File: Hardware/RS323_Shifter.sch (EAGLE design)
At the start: 16 parts, among them U2 XN04312

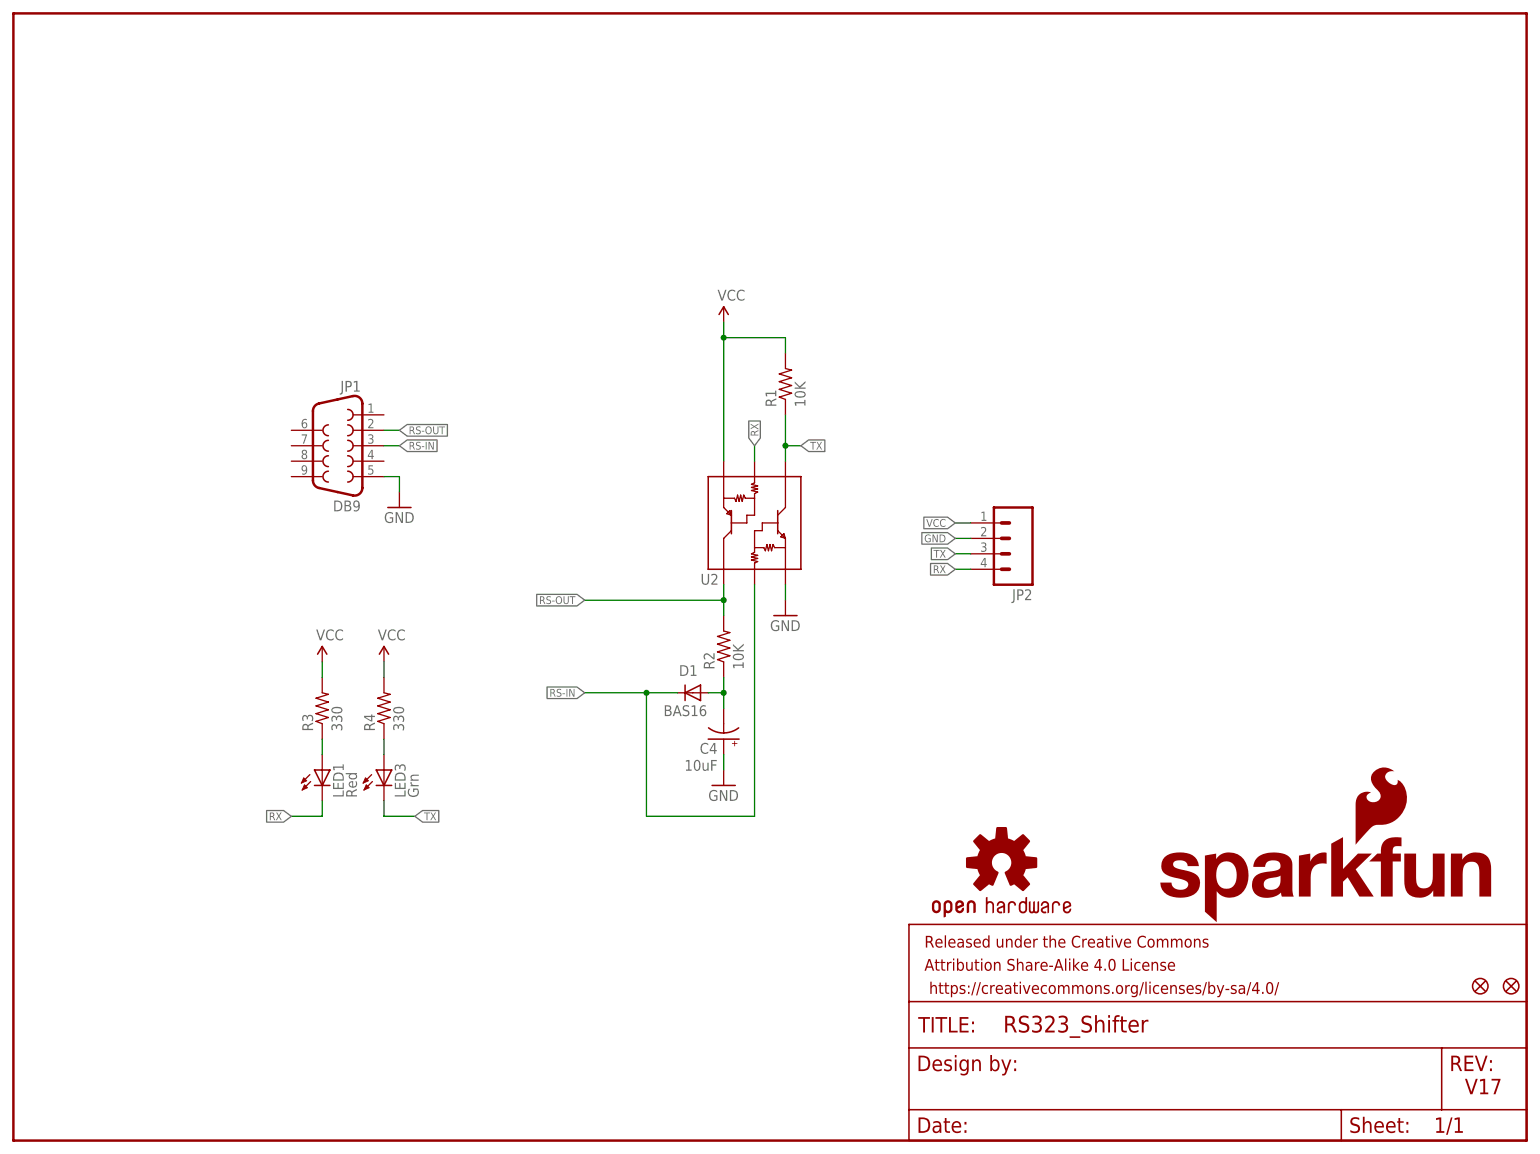
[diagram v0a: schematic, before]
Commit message: New files
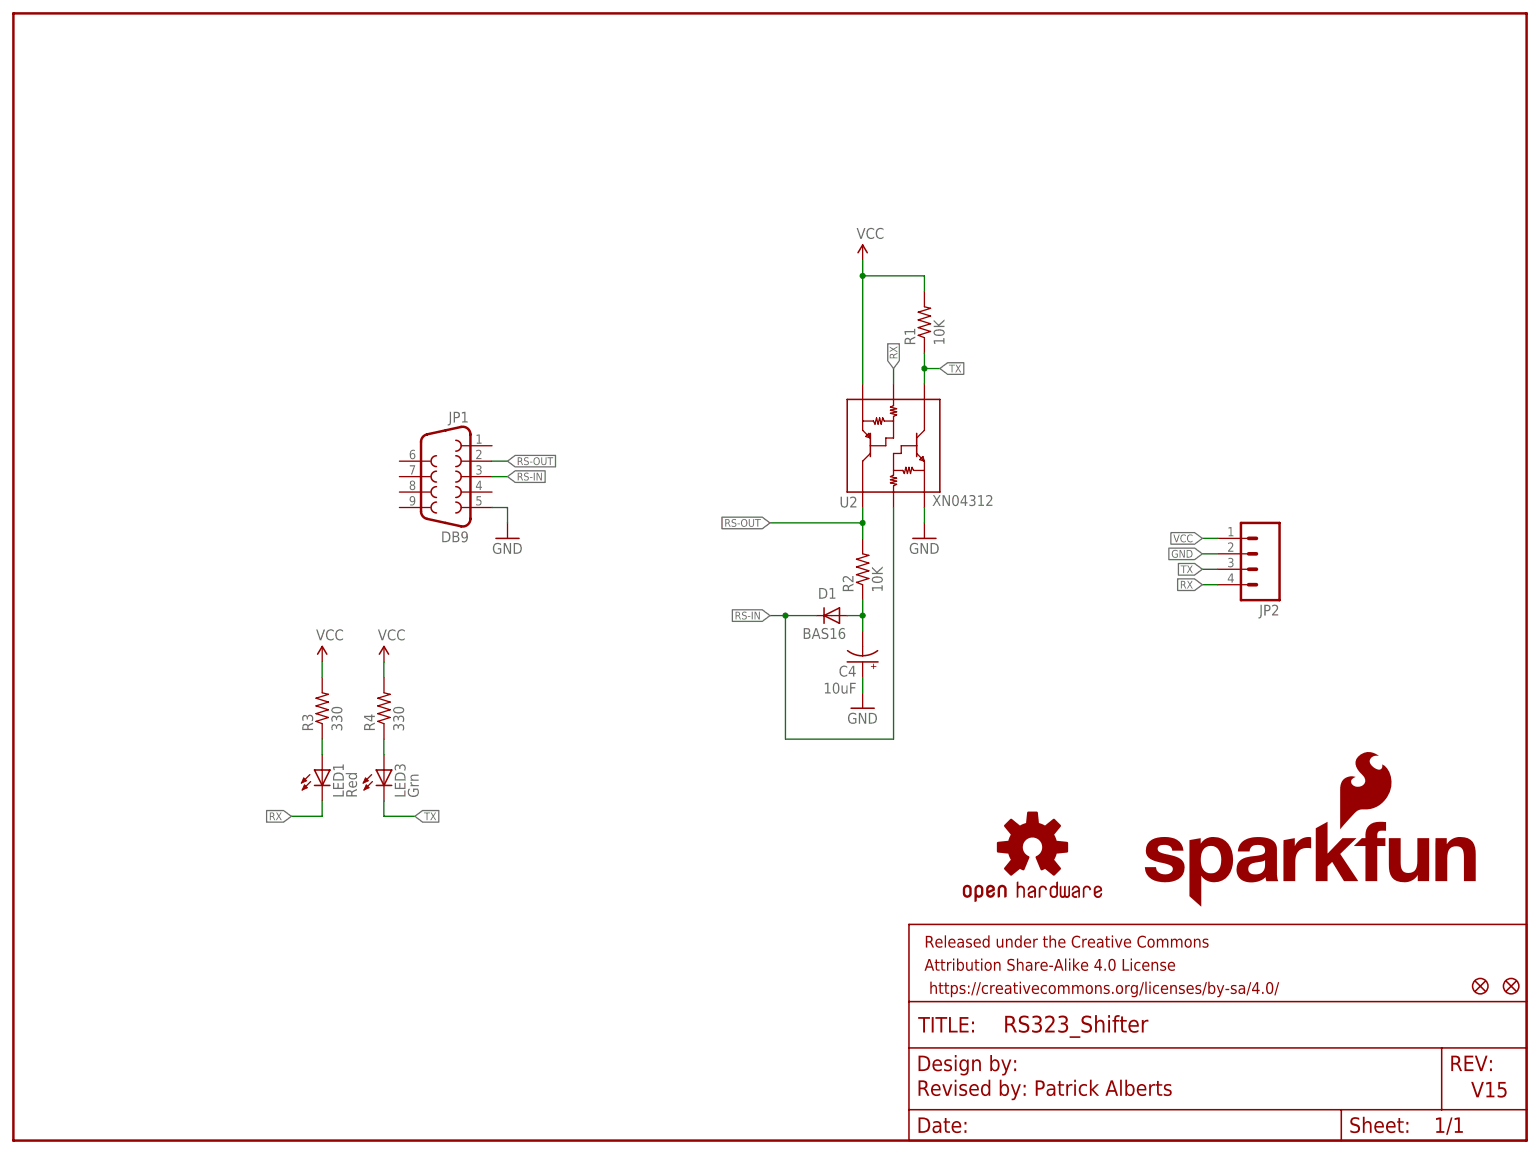
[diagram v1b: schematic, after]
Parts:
- JP1: device Testing:DB9L17SM209S114T -> SparkFun-Connectors:DB9FEMALE
- JP2: device SparkFun:M04PTH -> SparkFun-Connectors:M04LOCK
- LOGO1: value SFE_LOGO_NAME_FLAME.2_INCH -> SFE_LOGO_NAME_FLAME.1_INCH; device SparkFun-Aesthetics:SFE_LOGO_NAME_FLAME.2_INCH -> SparkFun-Aesthetics:SFE_LOGO_NAME_FLAME.1_INCH
- R1, R2: device SparkFun:RESISTOR0603-RES -> SparkFun-Resistors:10KOHM1/10W1%(0603)0603
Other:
- note added: "Revised by: Patrick Alberts"
- note added: "V15"
- note removed: "V17"
- moved on the sheet: C4, D1, JP1, JP2, R1, R2, U2
